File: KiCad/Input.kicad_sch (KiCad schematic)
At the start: 629 parts, among them J1 R_Phono_In, J10 VCC_IN, J11 VCC_OUT, J12 EMK_In, J13 EMK_Out, J14 EMK_Out, J15 Mic_Effekt_Out, J16 Mic_Effekt_Out, J17 Mic_Effekt_Out, J18 Mic_Effekt_Out, J19 Phono/Line_Out, J2 L_Phono_In, J20 Mic_Effekt_Out, J21 EMK_Out, J22 EMK_In, J23 EMK_In, J24 Mic_Effekt_In, J25 Mic_Effekt_In, J26 Phono/Line_In, J27 Mic_Effekt_In, J28 Pegel_Out, J29 Pegel_Out, J3 R_Line_In, J30 Pegel_In, J31 Pegel_In, J32 Pegel_In, J33 Pegel_In, J34 LED_Out, J35 LED_In, J36 VU_Meter_Out, J37 AUX_Send_3, J38 AUX_Send_1, J39 AUX_Send_2, J4 L_Line_In, J40 Bass_Out, J41 Kick_Out, J42 Mid_Out, J43 High_Out, J44 Line_Out_L, J45 Line_Out_R, J5 Mic_In, J6 Effekt_In, J7 AUX_RET_1, J8 AUX_RET_2, J9 AUX_RET_3, SW1 SW_DPST, SW10 SW_SPDT, SW11 SW_SPDT, SW12 SW_SPDT, SW2 SW_SPDT, SW3 SW_SPDT, SW4 SW_SPDT, SW5 SW_SPDT, SW6 SW_SPDT, SW7 SW_SPDT, SW8 SW_SPDT, SW9 Pegel_Selector, U1 TL074, U10 TL074, U11 TL074, U12 TL074, U13 TL074, U14 TL074, U15 TL074, U16 TL074, U17 TL074, U18 TL074, U19 TL074, U2 TL074, U20 TL074, U21 TL074, U22 TL074, U23 TL074, U24 TL074, U25 INA128U, U3 TL074, U4 TL074, U5 TL074, U6 REC10K-2409, U7 REC10K-2415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

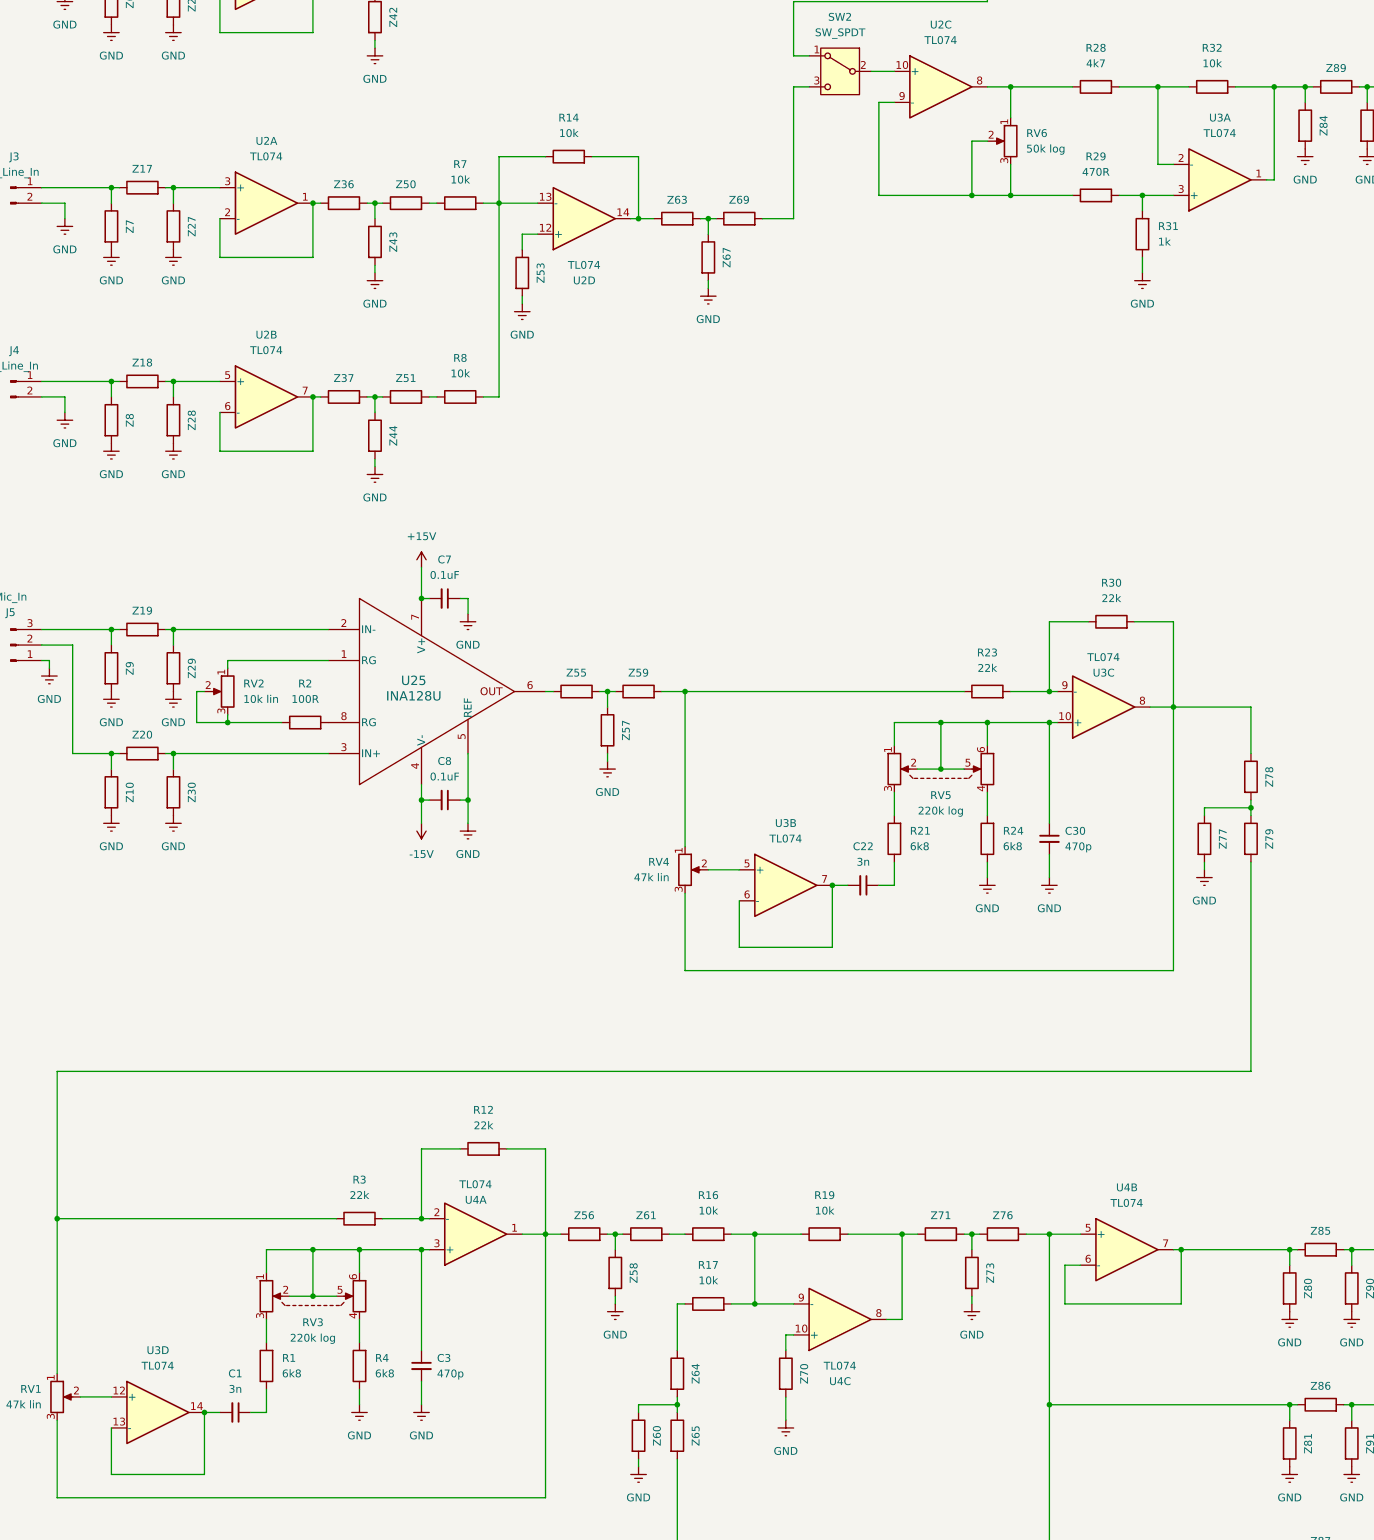
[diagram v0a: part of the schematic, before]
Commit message: PCB Update
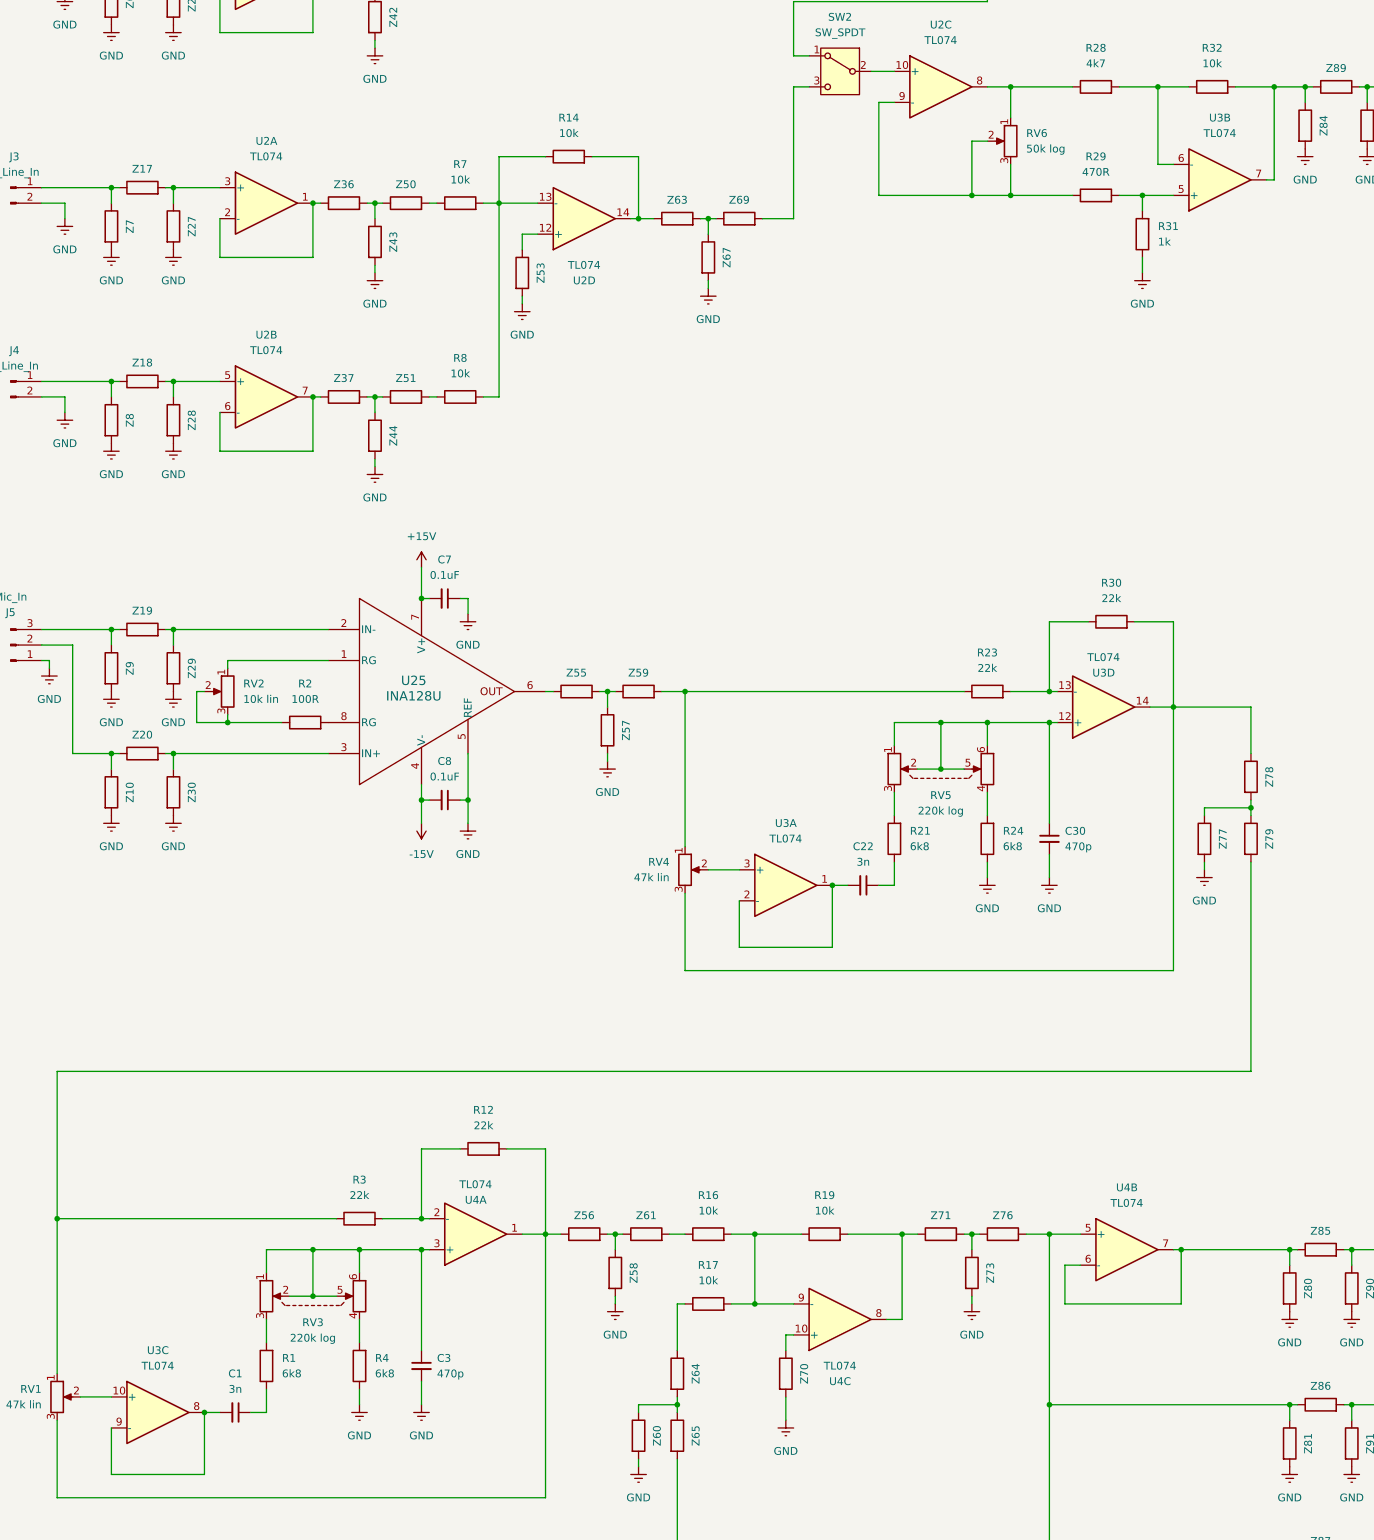
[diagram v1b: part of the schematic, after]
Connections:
- net at R29.2, R31.2: now also U3.5 (+); no longer U3.3 (+)
- net at R32.2, Z84.1, Z89.1: now also U3.7; no longer U3.1
- net at RV1.2: now also U3.10 (+); no longer U3.12 (+)
- net at C30.1, RV5.1, RV5.2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: now also U3.12 (+); no longer U3.10 (+)
- net at R30.2, RV4.3, Z78.1: now also U3.14; no longer U3.8
- net at R23.2, R30.1: now also U3.13 (-); no longer U3.9 (-)
- net at RV4.2: now also U3.3 (+); no longer U3.5 (+)
- net at R28.2, R32.1: now also U3.6 (-); no longer U3.2 (-)
- new net: C22.2, U3.1, U3.2 (-)
- new net: C1.2, U3.8, U3.9 (-)
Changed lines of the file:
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@@
 		(at 204.47 213.36 0)
 		(mirror x)
-		(unit 3)
+		(unit 4)
 		(exclude_from_sim no)
 		(in_bom yes)
@@
 				(path "/81a92cd6-862a-4567-ad33-f8a3bc120591"
 					(reference "U3")
-					(unit 3)
+					(unit 4)
 				)
 			)
@@
 		(lib_id "Amplifier_Operational:TL074")
 		(at 152.4 242.57 0)
-		(unit 2)
+		(unit 1)
 		(exclude_from_sim no)
 		(in_bom yes)
@@
 				(path "/81a92cd6-862a-4567-ad33-f8a3bc120591"
 					(reference "U3")
-					(unit 2)
+					(unit 1)
 				)
 			)
@@
 		(lib_id "Amplifier_Operational:TL074")
 		(at 49.53 328.93 0)
-		(unit 4)
+		(unit 3)
 		(exclude_from_sim no)
 		(in_bom yes)
@@
 				(path "/81a92cd6-862a-4567-ad33-f8a3bc120591"
 					(reference "U3")
-					(unit 4)
+					(unit 3)
 				)
 			)
@@
 		(at 223.52 127 0)
 		(mirror x)
-		(unit 1)
+		(unit 2)
 		(exclude_from_sim no)
 		(in_bom yes)
@@
 				(path "/81a92cd6-862a-4567-ad33-f8a3bc120591"
 					(reference "U3")
-					(unit 1)
+					(unit 2)
 				)
 			)
